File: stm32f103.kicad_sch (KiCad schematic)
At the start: 37 parts, among them J101 HIROSE TYPE C, J102 STLINK, J103 SHIELD, J104 EXTPWR, Q101 AO3400A, SW101 RESET, SW102 BOOT, U101 MT6835, U102 XC6206, U103 STM32F103, Y101 12MHz

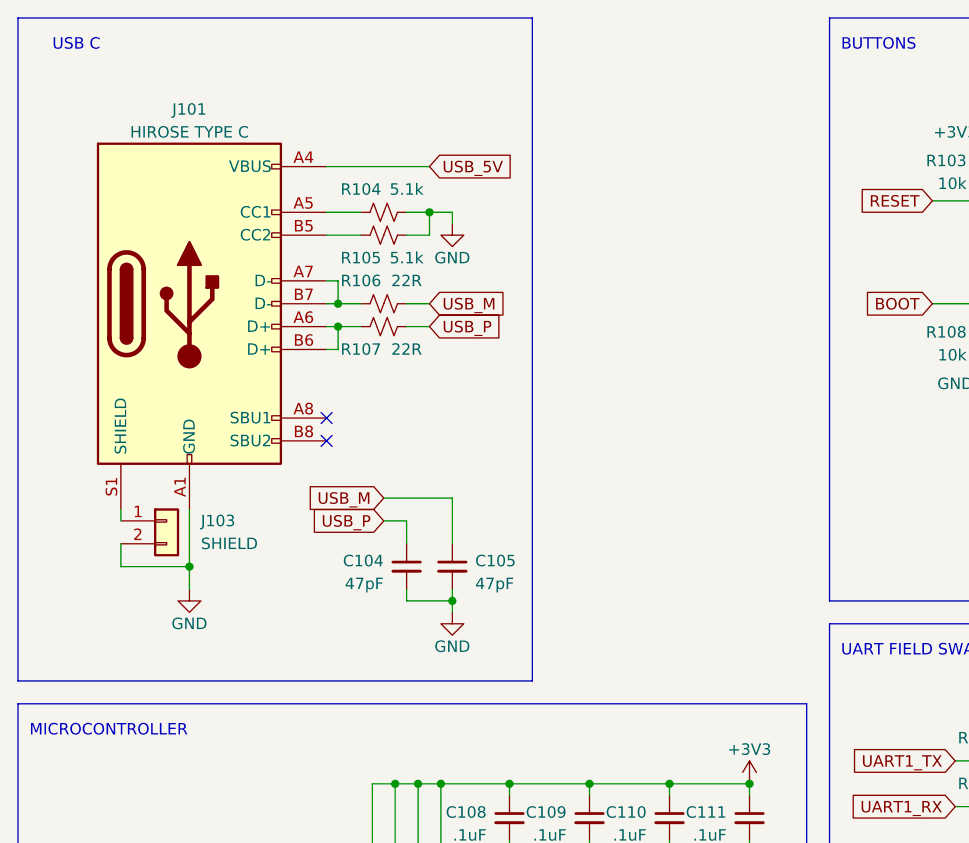
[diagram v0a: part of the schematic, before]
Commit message: add schematic pdf
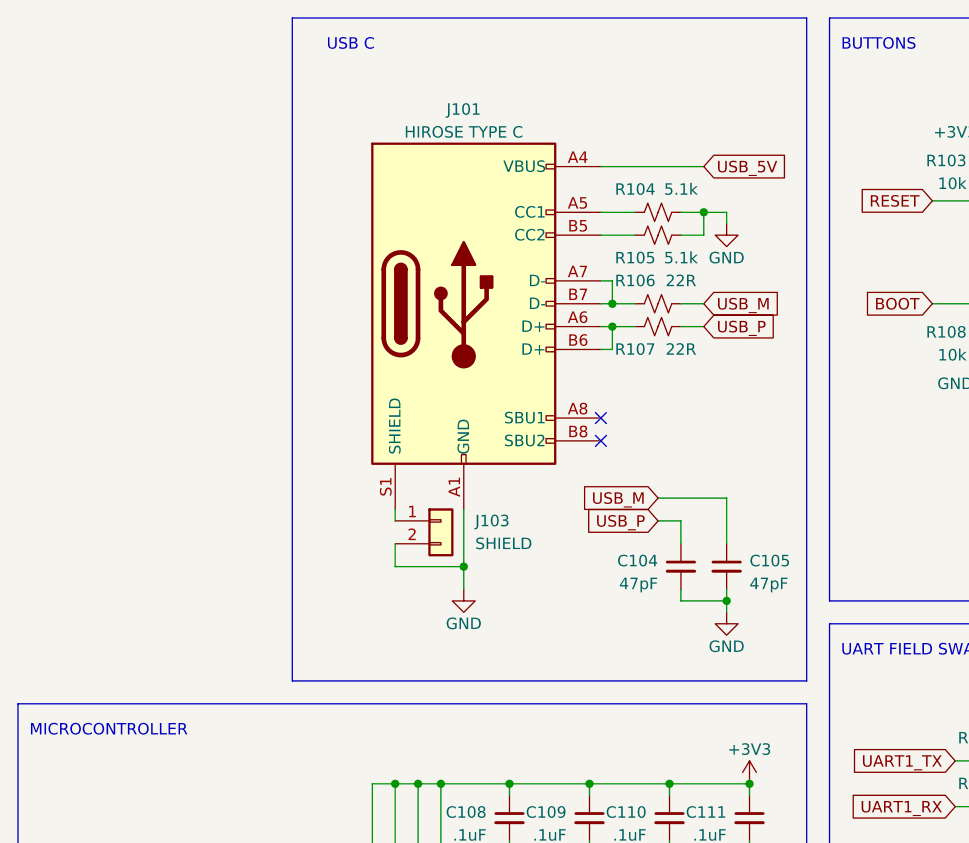
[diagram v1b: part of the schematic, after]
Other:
- moved on the sheet: C104, C105, J101, J103, R104, R105, R106, R107
